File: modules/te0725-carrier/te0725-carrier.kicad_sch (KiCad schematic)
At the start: 3 parts, among them J1 Conn_02x25_Odd_Even, J2 Conn_02x25_Odd_Even

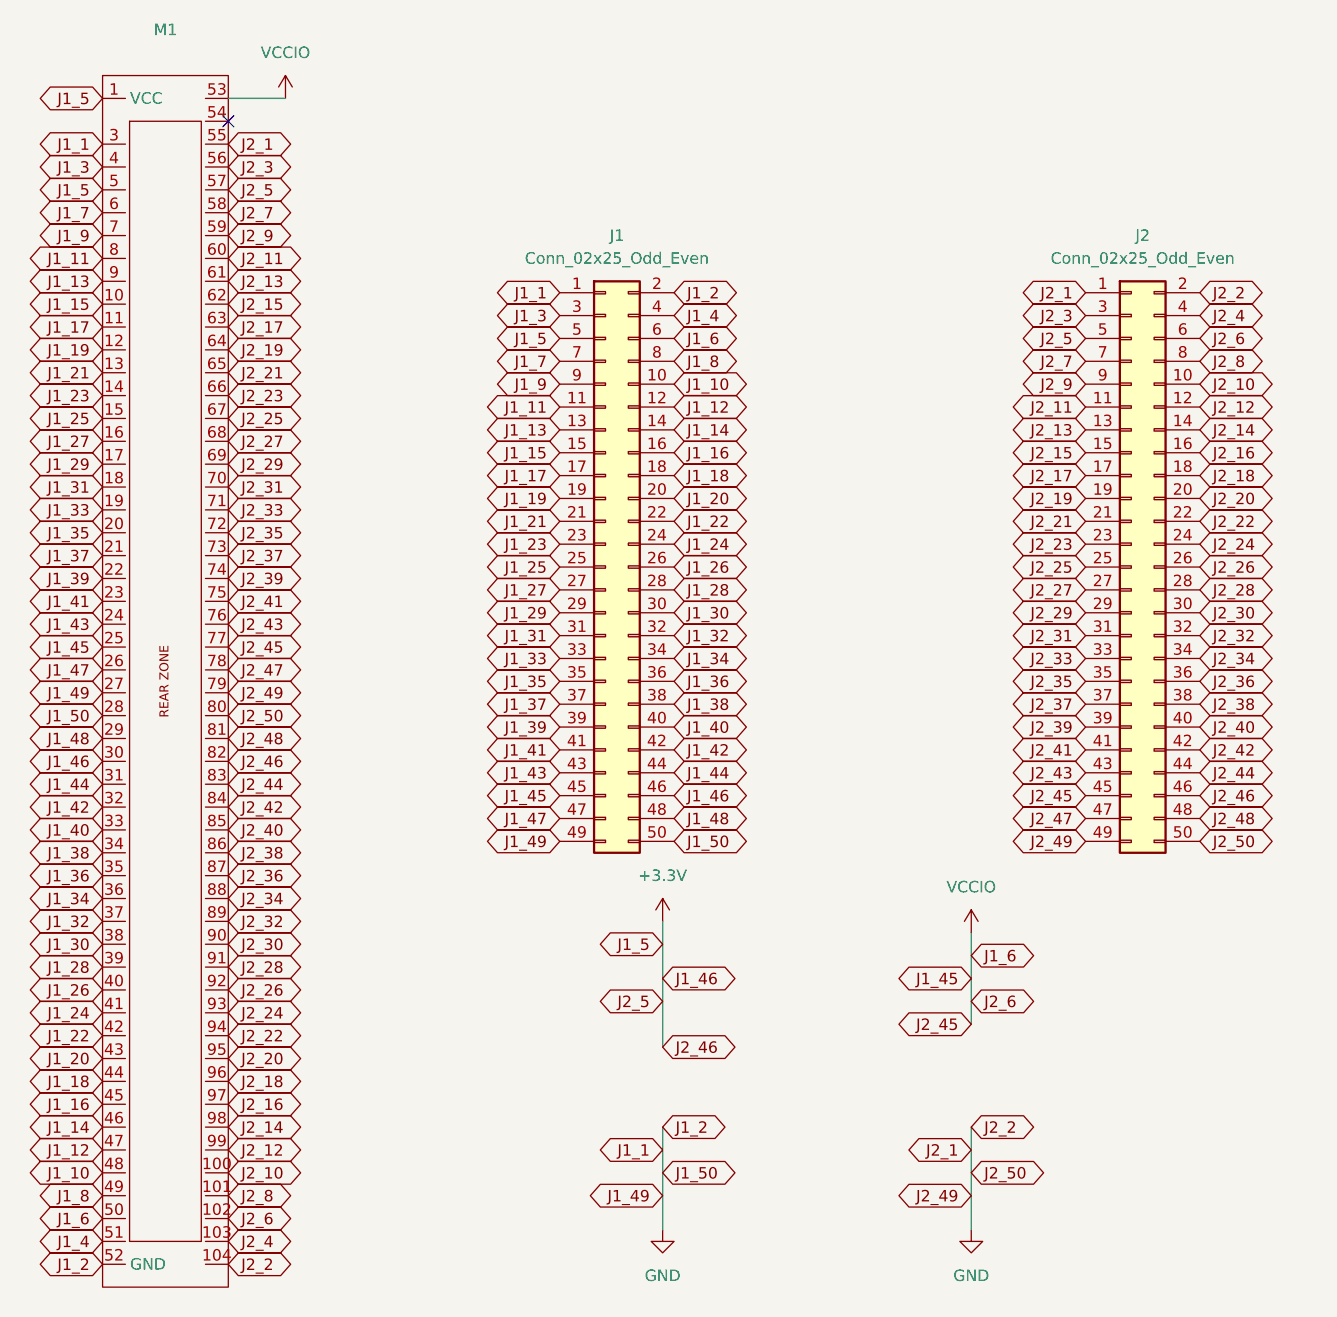
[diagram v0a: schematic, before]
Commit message: Updating all modules
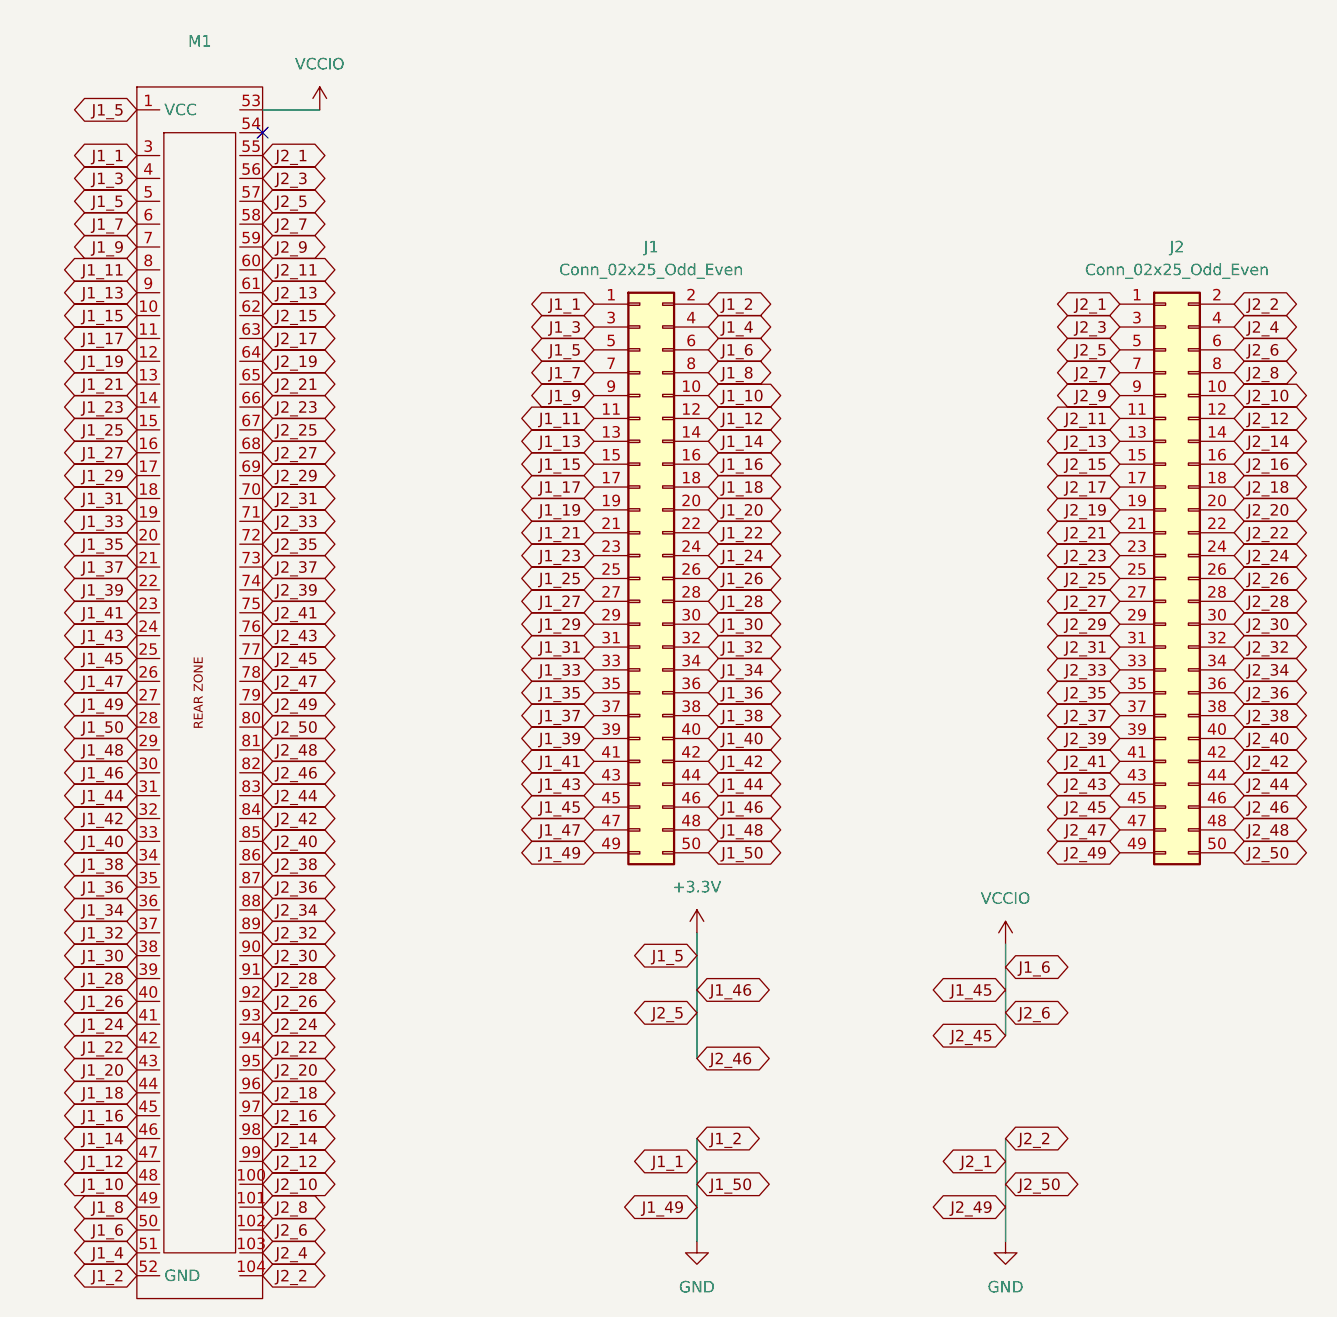
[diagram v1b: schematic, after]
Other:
- moved on the sheet: J1, J2, M1
